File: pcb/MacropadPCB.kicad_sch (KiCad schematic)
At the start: 27 parts, among them J1 Conn_01x04_Pin, SW1 SW_Push_45deg, SW2 SW_Push_45deg, SW3 SW_Push_45deg, SW4 SW_Push_45deg, SW5 SW_Push_45deg, SW6 SW_Push_45deg, U1 MOUDLE-SEEEDUINO-XIAO

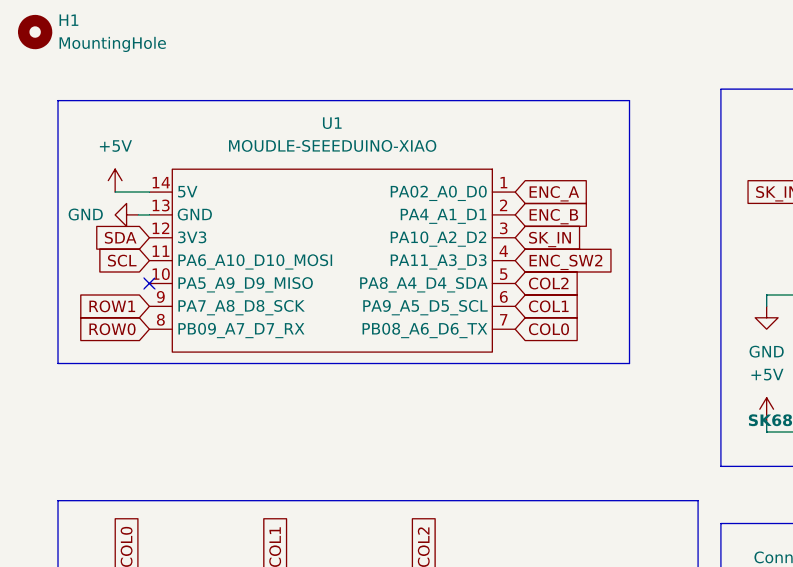
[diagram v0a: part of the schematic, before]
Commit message: Update project images and final documentation refinements
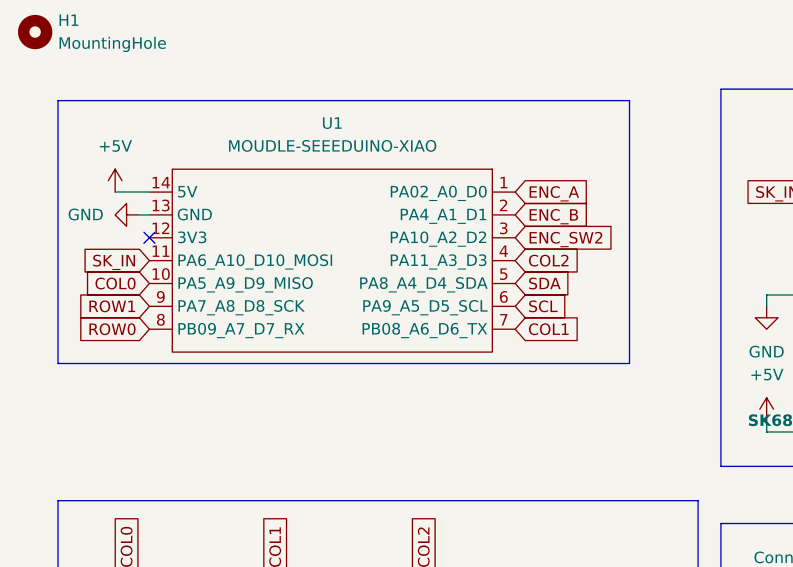
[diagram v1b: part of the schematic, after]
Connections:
- net COL0: now also U1.10 (PA5_A9_D9_MISO); no longer U1.7 (PB08_A6_D6_TX)
- net COL1: now also U1.7 (PB08_A6_D6_TX); no longer U1.6 (PA9_A5_D5_SCL)
- net COL2: now also U1.4 (PA11_A3_D3); no longer U1.5 (PA8_A4_D4_SDA)
- net ENC_SW2: now also U1.3 (PA10_A2_D2); no longer U1.4 (PA11_A3_D3)
- net SCL: now also U1.6 (PA9_A5_D5_SCL); no longer U1.11 (PA6_A10_D10_MOSI)
- net SDA: now also U1.5 (PA8_A4_D4_SDA); no longer U1.12 (3V3)
- net SK_IN: now also U1.11 (PA6_A10_D10_MOSI); no longer U1.3 (PA10_A2_D2)
